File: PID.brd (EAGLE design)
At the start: 67.3 x 40.3 mm, 32 parts, among them IC1 UA741CPE4, IC2 UA741CPE4, IC3 UA741CPE4, IC4 UA741CPE4, IC5 UA741CPE4

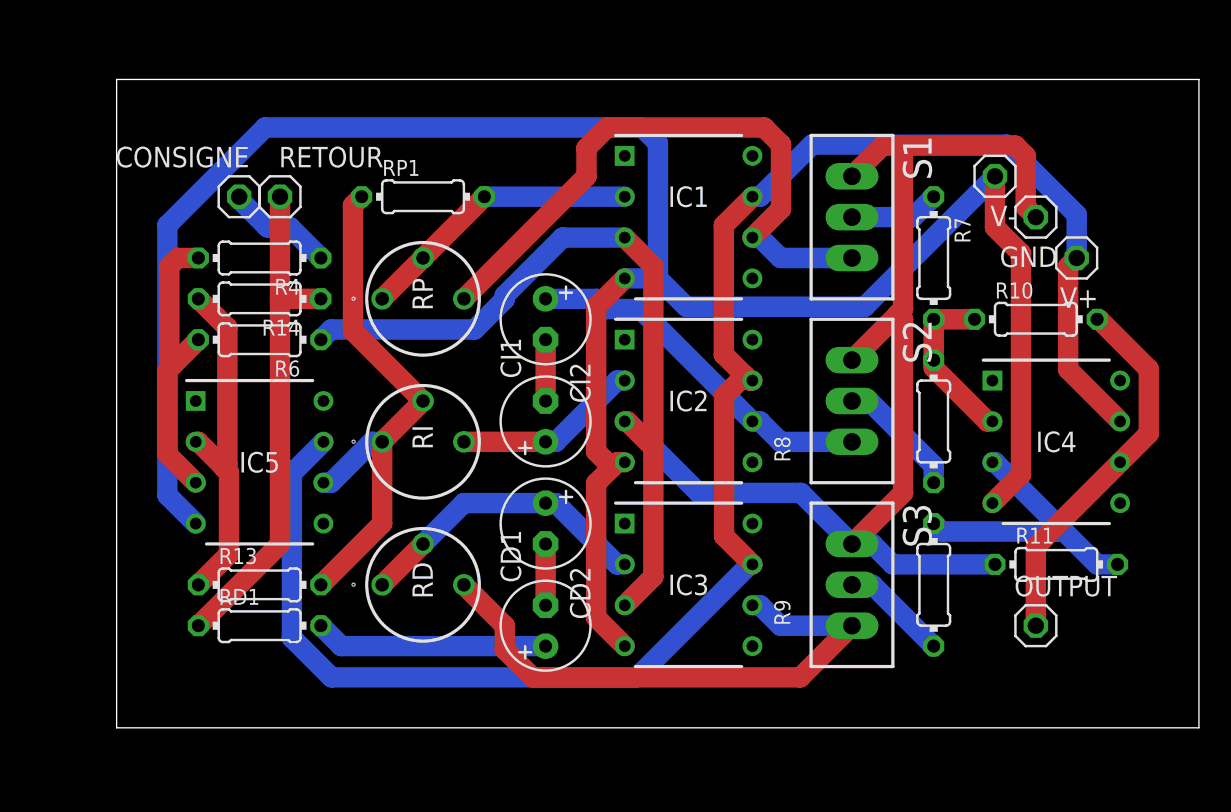
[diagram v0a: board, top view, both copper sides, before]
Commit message: couocu
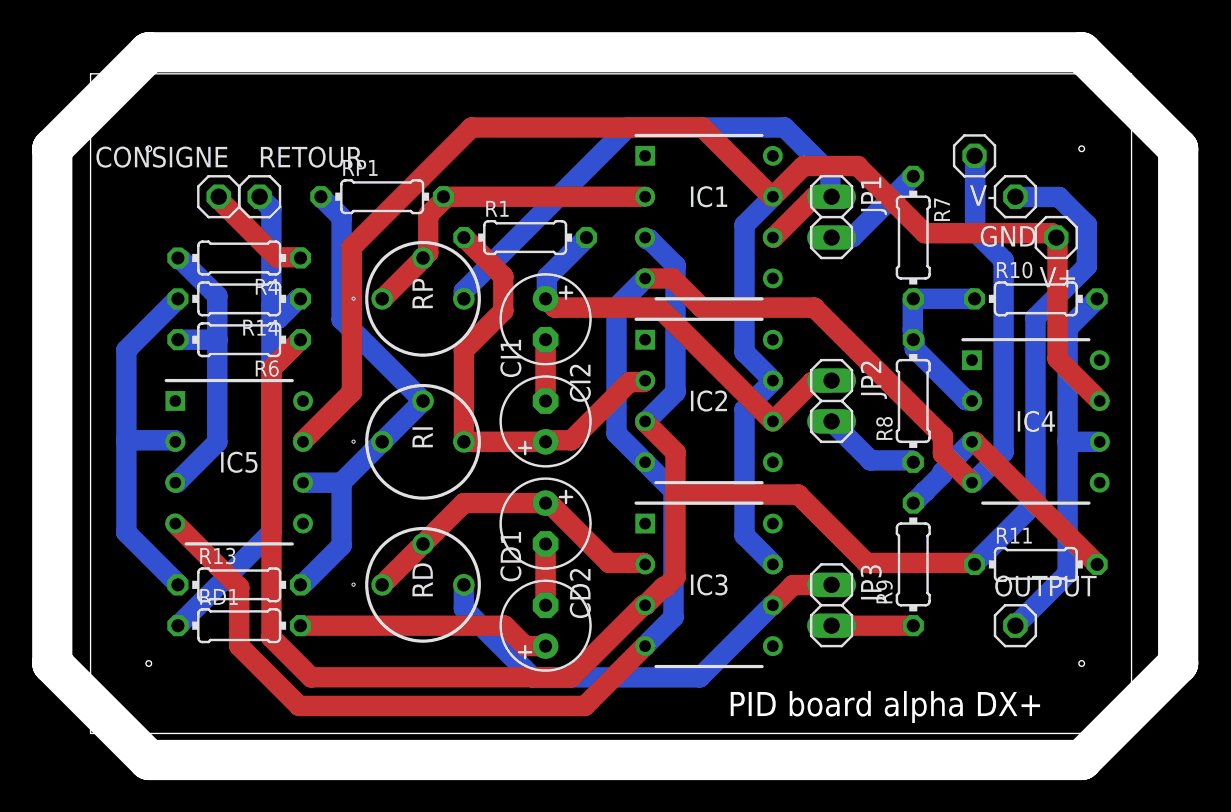
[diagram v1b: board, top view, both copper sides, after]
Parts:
- removed S1, S2, S3: TL36PO, switch:TL3XPO
- added JP1, JP2, JP3: (no value), pinhead:1X02
- added R1: 100k, rcl:0204/7
- moved RP1 2.54 mm to (16.5, 33.0)
- moved IC4 1.80 mm to (57.1, 19.1)
- moved GND 1.80 mm to (55.9, 33.0)
- moved V- 1.80 mm to (53.3, 35.6)
- moved R7 1.80 mm to (49.5, 30.5)
- moved R8 1.80 mm to (49.5, 20.3)
- moved R9 1.80 mm to (49.5, 10.2)
- moved V+ 1.80 mm to (58.4, 30.5)
- moved R10 1.27 mm to (57.1, 26.7)
- moved R11 1.27 mm to (57.1, 10.2)
- moved CONSIGNE 1.27 mm to (6.35, 33.0)
- moved IC5 1.27 mm to (7.62, 16.5)
- moved R13 1.27 mm to (7.62, 8.89)
- moved R14 1.27 mm to (7.62, 26.7)
- moved R4 1.27 mm to (7.62, 29.2)
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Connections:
- net N$15 renamed ERREUR
- net GND: no longer S1.1, S2.1, S3.1
- net N$10: now also JP3.1; no longer S3.3
- net N$12: now also JP1.2; no longer S1.2
- net N$16: now also JP2.2; no longer S2.2
- net N$19: now also JP3.2; no longer S3.2
- net N$2: now also JP1.1; no longer S1.3
- net N$4: now also JP2.1, R1.2; no longer S2.3
- net N$5: now also R1.1
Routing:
- net V-: track 136.0 -> 111.5 mm
- net N$5: track 11.6 -> 27.6 mm
- net V+: track 109.3 -> 101.7 mm
- net N$10: track 35.4 -> 28.5 mm
- net N$4: track 22.7 -> 26.8 mm
- net N$2: track 38.8 -> 34.8 mm
- net N$3: track 17.7 -> 20.5 mm
- net N$18: track 18.6 -> 16.3 mm
- net N$16: track 7.81 -> 6.13 mm
- net N$9: track 21.9 -> 23.6 mm
- net N$19: track 6.66 -> 5.08 mm
- net N$7: track 10.6 -> 11.9 mm
- net N$11: track 18.8 -> 20.0 mm
- net N$17: track 14.5 -> 15.8 mm
- net ERREUR: track 33.5 -> 32.4 mm
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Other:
- board size 67.3 x 40.3 mm -> 70 x 44 mm
- board text added: "PID board alpha DX+"
